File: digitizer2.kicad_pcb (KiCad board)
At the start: 2 copper layers, 3 parts, among them U1 XC7A35T, U3 MT41K128M16, U4 ADS5403

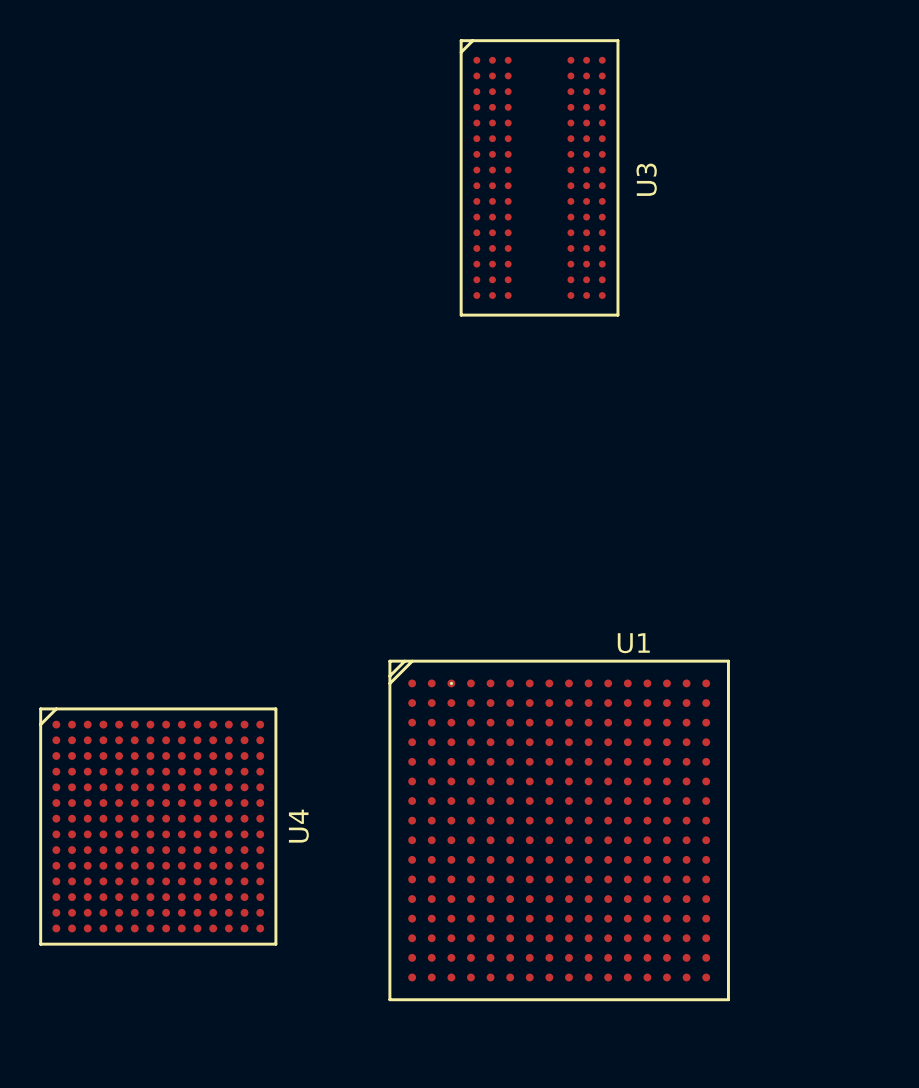
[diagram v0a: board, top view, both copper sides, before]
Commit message: Initial routing
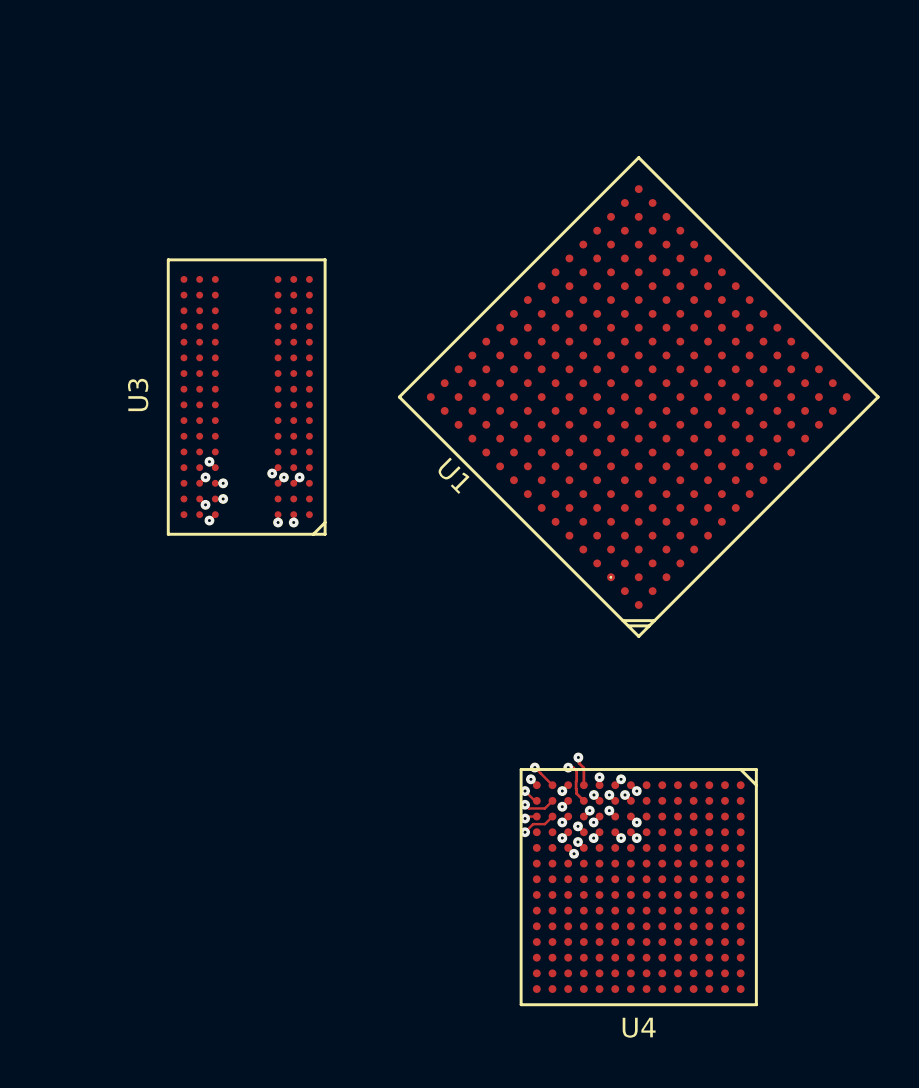
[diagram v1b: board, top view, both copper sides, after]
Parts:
- moved U4 24.7 mm to (160.0, 120.0), turned to 270 degrees
- moved U1 22.5 mm to (160.0, 95.0), turned to 135 degrees
- moved U3 18.7 mm to (140.0, 95.0), turned to 180 degrees
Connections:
- net Net-(U1-PadL7) renamed /JTAG_TCK
- net Net-(U1-PadM7) renamed /JTAG_TMS
- net Net-(U1-PadN7) renamed /JTAG_TDI
- net Net-(U1-PadN8) renamed /JTAG_TDO
- net Net-(U3-PadA2) renamed /DRAM_DQ13
- net Net-(U3-PadA3) renamed /DRAM_DQ15
- net Net-(U3-PadA7) renamed /DRAM_DQ12
- net Net-(U3-PadB7) renamed /DRAM_DQS1_N
- net Net-(U3-PadB8) renamed /DRAM_DQ14
- net Net-(U3-PadC2) renamed /DRAM_DQ11
- net Net-(U3-PadC3) renamed /DRAM_DQ9
- net Net-(U3-PadC7) renamed /DRAM_DQS1_P
- net Net-(U3-PadC8) renamed /DRAM_DQ10
- net Net-(U3-PadD3) renamed /DRAM_DM1
- net Net-(U3-PadD7) renamed /DRAM_DQ8
- net Net-(U3-PadE3) renamed /DRAM_DQ0
- net Net-(U3-PadE7) renamed /DRAM_DM0
- net Net-(U3-PadF2) renamed /DRAM_DQ2
- net Net-(U3-PadF3) renamed /DRAM_DQS0_P
- net Net-(U3-PadF7) renamed /DRAM_DQ1
- net Net-(U3-PadF8) renamed /DRAM_DQ3
- net Net-(U3-PadG2) renamed /DRAM_DQ6
- net Net-(U3-PadG3) renamed /DRAM_DQS0_N
- net Net-(U3-PadH3) renamed /DRAM_DQ4
- net Net-(U3-PadH7) renamed /DRAM_DQ7
- net Net-(U3-PadH8) renamed /DRAM_DQ5
- net Net-(U3-PadJ3) renamed /DRAM_RAS
- net Net-(U3-PadJ7) renamed /DRAM_CK_P
- net Net-(U3-PadK1) renamed /DRAM_ODT
- net Net-(U3-PadK3) renamed /DRAM_CAS
- net Net-(U3-PadK7) renamed /DRAM_CK_N
- net Net-(U3-PadK9) renamed /DRAM_CKE
- net Net-(U3-PadL2) renamed /DRAM_CS
- net Net-(U3-PadL3) renamed /DRAM_WE
- net Net-(U3-PadL7) renamed /DRAM_A10
- net Net-(U3-PadL8) renamed /DRAM_ZQ
- net Net-(U3-PadM2) renamed /DRAM_BA0
- net Net-(U3-PadM3) renamed /DRAM_BA2
- net Net-(U3-PadN2) renamed /DRAM_A3
- net Net-(U3-PadN3) renamed /DRAM_A0
- net Net-(U3-PadN7) renamed /DRAM_A12
- net Net-(U3-PadN8) renamed /DRAM_BA1
- net Net-(U3-PadP2) renamed /DRAM_A5
- net Net-(U3-PadP3) renamed /DRAM_A2
- net Net-(U3-PadP7) renamed /DRAM_A1
- net Net-(U3-PadP8) renamed /DRAM_A4
- net Net-(U3-PadR2) renamed /DRAM_A7
- net Net-(U3-PadR3) renamed /DRAM_A9
- net Net-(U3-PadR7) renamed /DRAM_A11
- net Net-(U3-PadR8) renamed /DRAM_A6
- net Net-(U3-PadT2) renamed /DRAM_RESET
- net Net-(U3-PadT3) renamed /DRAM_A13
- net Net-(U3-PadT8) renamed /DRAM_A8
- net Net-(U4-PadA10) renamed /ADC_SDO
- net Net-(U4-PadA11) renamed /ADC_SDIO
- net Net-(U4-PadA12) renamed /ADC_SCLK
- net Net-(U4-PadA13) renamed /ADC_SDENB
- net Net-(U4-PadH1) renamed /ADC_DACLK_N
- net Net-(U4-PadH2) renamed /ADC_DACLK_P
- net Net-(U4-PadH3) renamed /ADC_DA0_N
- net Net-(U4-PadH4) renamed /ADC_DA0_P
- net Net-(U4-PadJ1) renamed /ADC_DA1_N
- net Net-(U4-PadJ2) renamed /ADC_DA1_P
- net Net-(U4-PadJ3) renamed /ADC_DA2_N
- net Net-(U4-PadJ4) renamed /ADC_DA2_P
- net Net-(U4-PadK1) renamed /ADC_DA3_N
- net Net-(U4-PadK2) renamed /ADC_DA3_P
- net Net-(U4-PadK3) renamed /ADC_DA4_N
- net Net-(U4-PadK4) renamed /ADC_DA4_P
- net Net-(U4-PadL1) renamed /ADC_DA5_N
- net Net-(U4-PadL2) renamed /ADC_DA5_P
- net Net-(U4-PadL3) renamed /ADC_DA6_N
- net Net-(U4-PadL4) renamed /ADC_DA6_P
- net Net-(U4-PadL5) renamed /ADC_OVRA_N
- net Net-(U4-PadM1) renamed /ADC_DA7_N
- net Net-(U4-PadM2) renamed /ADC_DA7_P
- net Net-(U4-PadM3) renamed /ADC_DA8_N
- net Net-(U4-PadM4) renamed /ADC_DA8_P
- net Net-(U4-PadM5) renamed /ADC_OVRA_P
- net Net-(U4-PadN1) renamed /ADC_DA9_N
- net Net-(U4-PadN2) renamed /ADC_DA10_N
- net Net-(U4-PadN3) renamed /ADC_DA11_N
- net Net-(U4-PadP1) renamed /ADC_DA9_P
- net Net-(U4-PadP2) renamed /ADC_DA10_P
- net Net-(U4-PadP3) renamed /ADC_DA11_P
- U3 pad A8: Net-(U3-PadA8) -> Net-(U3-PadA1)
- U3 pad B3: Net-(U3-PadB3) -> Net-(U3-PadA9)
- U3 pad B9: Net-(U3-PadB9) -> Net-(U3-PadB1)
- U3 pad C1: Net-(U3-PadC1) -> Net-(U3-PadA1)
- U3 pad C9: Net-(U3-PadC9) -> Net-(U3-PadA1)
- U3 pad D1: Net-(U3-PadD1) -> Net-(U3-PadB1)
- U3 pad D2: Net-(U3-PadD2) -> Net-(U3-PadA1)
- U3 pad D8: Net-(U3-PadD8) -> Net-(U3-PadB1)
- U3 pad D9: Net-(U3-PadD9) -> Net-(U3-PadB2)
- U3 pad E1: Net-(U3-PadE1) -> Net-(U3-PadA9)
- U3 pad E2: Net-(U3-PadE2) -> Net-(U3-PadB1)
- U3 pad E8: Net-(U3-PadE8) -> Net-(U3-PadB1)
- U3 pad E9: Net-(U3-PadE9) -> Net-(U3-PadA1)
- U3 pad F1: Net-(U3-PadF1) -> Net-(U3-PadA1)
- U3 pad F9: Net-(U3-PadF9) -> Net-(U3-PadB1)
- U3 pad G1: Net-(U3-PadG1) -> Net-(U3-PadB1)
- U3 pad G7: Net-(U3-PadG7) -> Net-(U3-PadB2)
- U3 pad G8: Net-(U3-PadG8) -> Net-(U3-PadA9)
- U3 pad G9: Net-(U3-PadG9) -> Net-(U3-PadB1)
- U3 pad H2: Net-(U3-PadH2) -> Net-(U3-PadA1)
- U3 pad H9: Net-(U3-PadH9) -> Net-(U3-PadA1)
- U3 pad J2: Net-(U3-PadJ2) -> Net-(U3-PadA9)
- U3 pad J8: Net-(U3-PadJ8) -> Net-(U3-PadA9)
- U3 pad K2: Net-(U3-PadK2) -> Net-(U3-PadB2)
- U3 pad K8: Net-(U3-PadK8) -> Net-(U3-PadB2)
- U3 pad M1: Net-(U3-PadM1) -> Net-(U3-PadA9)
- U3 pad M9: Net-(U3-PadM9) -> Net-(U3-PadA9)
- U3 pad N1: Net-(U3-PadN1) -> Net-(U3-PadB2)
- U3 pad N9: Net-(U3-PadN9) -> Net-(U3-PadB2)
- U3 pad P1: Net-(U3-PadP1) -> Net-(U3-PadA9)
- U3 pad P9: Net-(U3-PadP9) -> Net-(U3-PadA9)
- U3 pad R1: Net-(U3-PadR1) -> Net-(U3-PadB2)
- U3 pad R9: Net-(U3-PadR9) -> Net-(U3-PadB2)
- U3 pad T1: Net-(U3-PadT1) -> Net-(U3-PadA9)
- U3 pad T9: Net-(U3-PadT9) -> Net-(U3-PadA9)
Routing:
- net /DRAM_DQ8: track 0.00 -> 20.3 mm, vias 0 -> 1
- net /DRAM_DQ10: track 0.00 -> 18.8 mm, vias 0 -> 1
- net /DRAM_DQ12: track 0.00 -> 17.6 mm, vias 0 -> 1
- net /DRAM_DQS1_N: track 0.00 -> 17.3 mm, vias 0 -> 1
- net /DRAM_DQ14: track 0.00 -> 17.2 mm, vias 0 -> 1
- net /DRAM_DQS1_P: track 0.00 -> 16.8 mm, vias 0 -> 1
- net /DRAM_DQ13: track 0.00 -> 15.7 mm, vias 0 -> 1
- net /DRAM_DQ15: track 0.00 -> 15.7 mm, vias 0 -> 1
- net /ADC_DA4_P: track 0.00 -> 14.9 mm, vias 0 -> 1
- net /ADC_DA4_N: track 0.00 -> 14.3 mm, vias 0 -> 1
- net /ADC_OVRA_P: track 0.00 -> 13.9 mm, vias 0 -> 1
- net /ADC_DA2_P: track 0.00 -> 13.7 mm, vias 0 -> 1
- net /ADC_DA0_P: track 0.00 -> 13.6 mm, vias 0 -> 1
- net /ADC_OVRA_N: track 0.00 -> 13.6 mm, vias 0 -> 1
- net /ADC_DA11_N: track 0.00 -> 13.1 mm, vias 0 -> 1
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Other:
- copper layers 2 -> 6
- net class Default: clearance 0.2 -> 0.125; trace_width 0.25 -> 0.13; via_dia 0.6 -> 0.5; via_drill 0.4 -> 0.15
- rule pad_to_mask_clearance: 0.2 -> 0.05
- rule trace_clearance: 0.2 -> 0.125
- rule trace_min: 0.2 -> 0.125
- rule via_min_drill: 0.3 -> 0.15
- rule via_min_size: 0.4 -> 0.5
